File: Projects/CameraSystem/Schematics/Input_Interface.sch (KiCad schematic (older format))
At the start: 0 parts

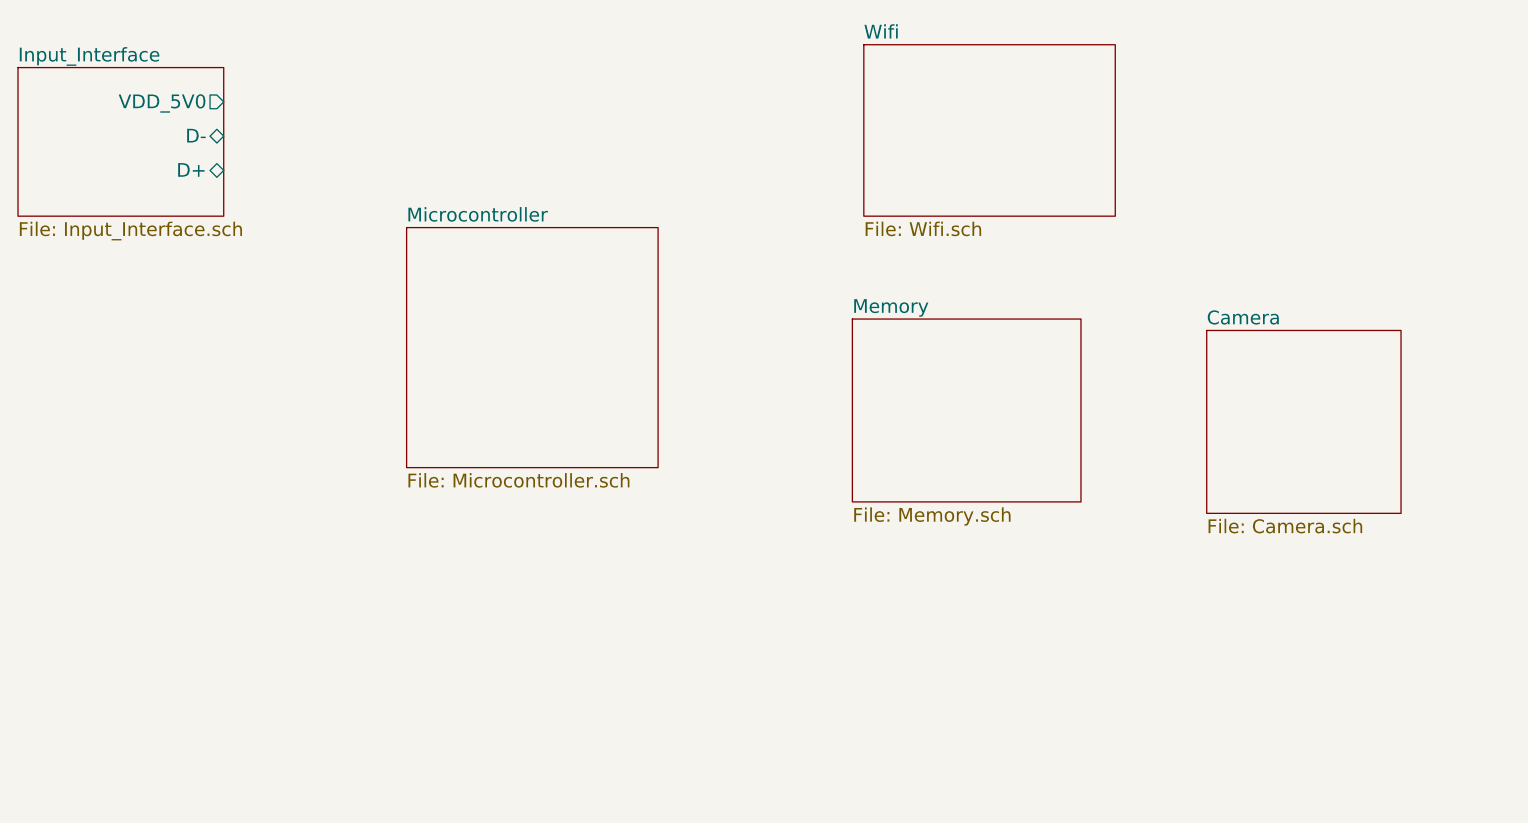
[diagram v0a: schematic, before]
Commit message: feat: set up layout
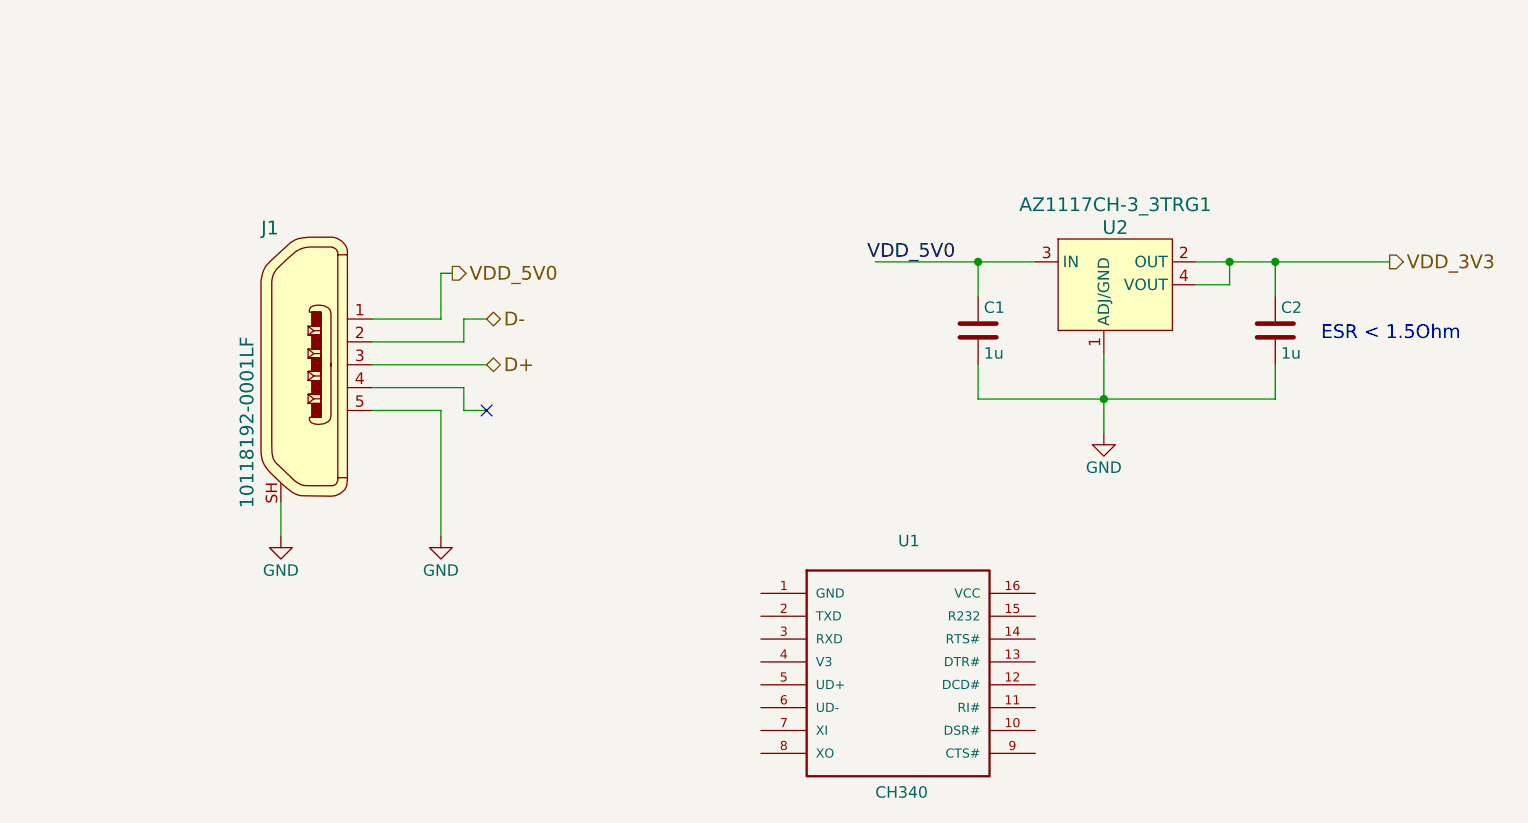
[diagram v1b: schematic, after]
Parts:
- added C1, C2: 1u, Capacitors_SMD:C_0603_HandSoldering, symbol C
- added J1: 10118192-0001LF, digikey-footprints:USB_Micro_B_Female_10118192, symbol 10118192-0001LF
- added U1: CH340, custom-footprints:SO16, symbol CH340
- added U2: AZ1117CH-3_3TRG1, digikey-footprints:SOT-223, symbol AZ1117CH-3_3TRG1
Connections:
- net labels added: D+, D-, GND, VDD_3V3, VDD_5V0
- wire segments 0 -> 23
- no-connect marks 0 -> 1
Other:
- note added: "ESR < 1.5Ohm"
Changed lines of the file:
@@
 $Descr A4 11693 8268
 encoding utf-8
-Sheet 1 6
+Sheet 2 6
 Title ""
 Date ""
@@
 Comment4 ""
 $EndDescr
-$Sheet
-S 1000 1000 900  650
-U 5BB4C1AE
-F0 "Input_Interface" 60
-F1 "Input_Interface.sch" 60
-F2 "VDD_5V0" O R 1900 1150 60
-F3 "D-" B R 1900 1300 60
-F4 "D+" B R 1900 1450 60
-$EndSheet
-$Sheet
-S 2700 1700 1100 1050
-U 5BB4D99F
-F0 "Microcontroller" 60
-F1 "Microcontroller.sch" 60
-$EndSheet
-$Sheet
-S 4700 900  1100 750
-U 5BB4D9C1
-F0 "Wifi" 60
-F1 "Wifi.sch" 60
-$EndSheet
-$Sheet
-S 4650 2100 1000 800
-U 5BB4DA56
-F0 "Memory" 60
-F1 "Memory.sch" 60
-$EndSheet
-$Sheet
-S 6200 2150 850  800
-U 5BB4DA63
-F0 "Camera" 60
-F1 "Camera.sch" 60
-$EndSheet
+$Comp
+L 10118192-0001LF J1
+U 1 1 5BB4C296
+P 2250 2300
+F 0 "J1" H 2102 2898 60  0000 C CNN
+F 1 "10118192-0001LF" V 2002 2048 60  0000 C CNN
+F 2 "digikey-footprints:USB_Micro_B_Female_10118192" H 2450 2500 60  0001 L CNN
+F 3 "https://cdn.amphenol-icc.com/media/wysiwyg/files/drawing/10118192.pdf" H 2450 2600 60  0001 L CNN
+F 4 "609-4613-1-ND" H 2450 2700 60  0001 L CNN "Digi-Key_PN"
+F 5 "10118192-0001LF" H 2450 2800 60  0001 L CNN "MPN"
+F 6 "Connectors, Interconnects" H 2450 2900 60  0001 L CNN "Category"
+F 7 "USB, DVI, HDMI Connectors" H 2450 3000 60  0001 L CNN "Family"
+F 8 "https://cdn.amphenol-icc.com/media/wysiwyg/files/drawing/10118192.pdf" H 2450 3100 60  0001 L CNN "DK_Datasheet_Link"
+F 9 "/product-detail/en/amphenol-fci/10118192-0001LF/609-4613-1-ND/2785378" H 2450 3200 60  0001 L CNN "DK_Detail_Page"
+F 10 "CONN USB MICRO B RECPT SMT R/A" H 2450 3300 60  0001 L CNN "Description"
+F 11 "Amphenol FCI" H 2450 3400 60  0001 L CNN "Manufacturer"
+F 12 "Active" H 2450 3500 60  0001 L CNN "Status"
+	1    2250 2300
+	1    0    0    -1
+$EndComp
+Wire Wire Line
+	2550 2100 2850 2100
+Wire Wire Line
+	2850 2100 2850 1900
+Wire Wire Line
+	2850 1900 2900 1900
+$Comp
+L GND #PWR01
+U 1 1 5BB4C3EB
+P 2850 3050
+F 0 "#PWR01" H 2850 2800 50  0001 C CNN
+F 1 "GND" H 2850 2900 50  0000 C CNN
+F 2 "" H 2850 3050 50  0001 C CNN
+F 3 "" H 2850 3050 50  0001 C CNN
+	1    2850 3050
+	1    0    0    -1
+$EndComp
+Wire Wire Line
+	2550 2500 2850 2500
+Wire Wire Line
+	2850 2500 2850 3050
+Wire Wire Line
+	2550 2200 2950 2200
+Wire Wire Line
+	2950 2200 2950 2100
+Wire Wire Line
+	2950 2100 3050 2100
+Wire Wire Line
+	2550 2300 3050 2300
+Wire Wire Line
+	2550 2400 2950 2400
+NoConn ~ 3050 2500
+Wire Wire Line
+	2950 2400 2950 2500
+Wire Wire Line
+	2950 2500 3050 2500
+$Comp
+L GND #PWR02
+U 1 1 5BB4C4E7
+P 2150 3050
+F 0 "#PWR02" H 2150 2800 50  0001 C CNN
+F 1 "GND" H 2150 2900 50  0000 C CNN
+F 2 "" H 2150 3050 50  0001 C CNN
+F 3 "" H 2150 3050 50  0001 C CNN
+	1    2150 3050
+	1    0    0    -1
+$EndComp
+Wire Wire Line
+	2150 2900 2150 3050
+Text HLabel 2900 1900 2    60   Output ~ 0
+VDD_5V0
+Text HLabel 3050 2100 2    60   BiDi ~ 0
+D-
+Text HLabel 3050 2300 2    60   BiDi ~ 0
+D+
+$Comp
+L AZ1117CH-3_3TRG1 U2
+U 1 1 5BB4D847
+P 5750 1850
+F 0 "U2" H 5800 2000 60  0000 C CNN
+F 1 "AZ1117CH-3_3TRG1" H 5800 2100 60  0000 C CNN
+F 2 "digikey-footprints:SOT-223" H 5950 2050 60  0001 L CNN
+F 3 "https://www.diodes.com/assets/Datasheets/AZ1117C.pdf" H 5950 2150 60  0001 L CNN
+F 4 "AZ1117CH-3.3TRG1DICT-ND" H 5950 2250 60  0001 L CNN "Digi-Key_PN"
+F 5 "AZ1117CH-3.3TRG1" H 5950 2350 60  0001 L CNN "MPN"
+F 6 "Integrated Circuits (ICs)" H 5950 2450 60  0001 L CNN "Category"
+F 7 "PMIC - Voltage Regulators - Linear" H 5950 2550 60  0001 L CNN "Family"
+F 8 "https://www.diodes.com/assets/Datasheets/AZ1117C.pdf" H 5950 2650 60  0001 L CNN "DK_Datasheet_Link"
+F 9 "/product-detail/en/diodes-incorporated/AZ1117CH-3.3TRG1/AZ1117CH-3.3TRG1DICT-ND/4505206" H 5950 2750 60  0001 L CNN "DK_Detail_Page"
+F 10 "IC REG LINEAR 3.3V 800MA SOT223" H 5950 2850 60  0001 L CNN "Description"
+F 11 "Diodes Incorporated" H 5950 2950 60  0001 L CNN "Manufacturer"
+F 12 "Active" H 5950 3050 60  0001 L CNN "Status"
+	1    5750 1850
+	1    0    0    -1
+$EndComp
+$Comp
+L CH340 U1
+U 1 1 5BB4DB29
+P 4850 3600
+F 0 "U1" H 4850 4100 50  0000 L BNN
+F 1 "CH340" H 4750 3000 50  0000 L BNN
+F 2 "custom-footprints:SO16" H 4750 3250 50  0001 L BNN
+F 3 "Fram" H 4800 3500 50  0001 L BNN
+	1    4850 3600
+	1    0    0    -1
+$EndComp
+Wire Wire Line
+	4750 1850 5450 1850
+Text Label 5100 1850 2    60   ~ 0
+VDD_5V0
+$Comp
+L GND #PWR03
+U 1 1 5BB4DDE6
+P 5750 2600
+F 0 "#PWR03" H 5750 2350 50  0001 C CNN
+F 1 "GND" H 5750 2450 50  0000 C CNN
+F 2 "" H 5750 2600 50  0001 C CNN
+F 3 "" H 5750 2600 50  0001 C CNN
+	1    5750 2600
+	1    0    0    -1
+$EndComp
+Wire Wire Line
+	5750 2250 5750 2600
+Wire Wire Line
+	6150 1950 6300 1950
+Wire Wire Line
+	6300 1950 6300 1850
+Wire Wire Line
+	6150 1850 7000 1850
+Connection ~ 6300 1850
+Text HLabel 7000 1850 2    60   Output ~ 0
+VDD_3V3
+$Comp
+L C C1
+U 1 1 5BB4E02C
+P 5200 2150
+F 0 "C1" H 5225 2250 50  0000 L CNN
+F 1 "1u" H 5225 2050 50  0000 L CNN
+F 2 "Capacitors_SMD:C_0603_HandSoldering" H 5238 2000 50  0001 C CNN
+F 3 "" H 5200 2150 50  0001 C CNN
+	1    5200 2150
+	1    0    0    -1
+$EndComp
+$Comp
+L C C2
+U 1 1 5BB4E099
+P 6500 2150
+F 0 "C2" H 6525 2250 50  0000 L CNN
+F 1 "1u" H 6525 2050 50  0000 L CNN
+F 2 "Capacitors_SMD:C_0603_HandSoldering" H 6538 2000 50  0001 C CNN
+F 3 "" H 6500 2150 50  0001 C CNN
+	1    6500 2150
+	1    0    0    -1
+$EndComp
+Text Notes 6700 2200 0    60   ~ 0
+ESR < 1.5Ohm
+Wire Wire Line
+	5200 2000 5200 1850
+Connection ~ 5200 1850
+Wire Wire Line
+	5200 2300 5200 2450
+Wire Wire Line
+	5200 2450 6500 2450
+Connection ~ 5750 2450
+Wire Wire Line
+	6500 2450 6500 2300
+Wire Wire Line
+	6500 2000 6500 1850
+Connection ~ 6500 1850
 $EndSCHEMATC
